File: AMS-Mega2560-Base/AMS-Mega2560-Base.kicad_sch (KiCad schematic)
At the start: 19 parts, among them J1 RTD1, J2 RTD2, J3 AdafruitUltimateGPS, J4 Sense, J5 Sense, P1 Power, P10 CONN_01X01, P11 CONN_01X01, P12 CONN_01X01, P13 CONN_01X01, P2 Analog, P3 Analog, P4 Digital, P5 PWM, P6 PWM, P7 Communication, P8 CONN_01X01, P9 CONN_01X01

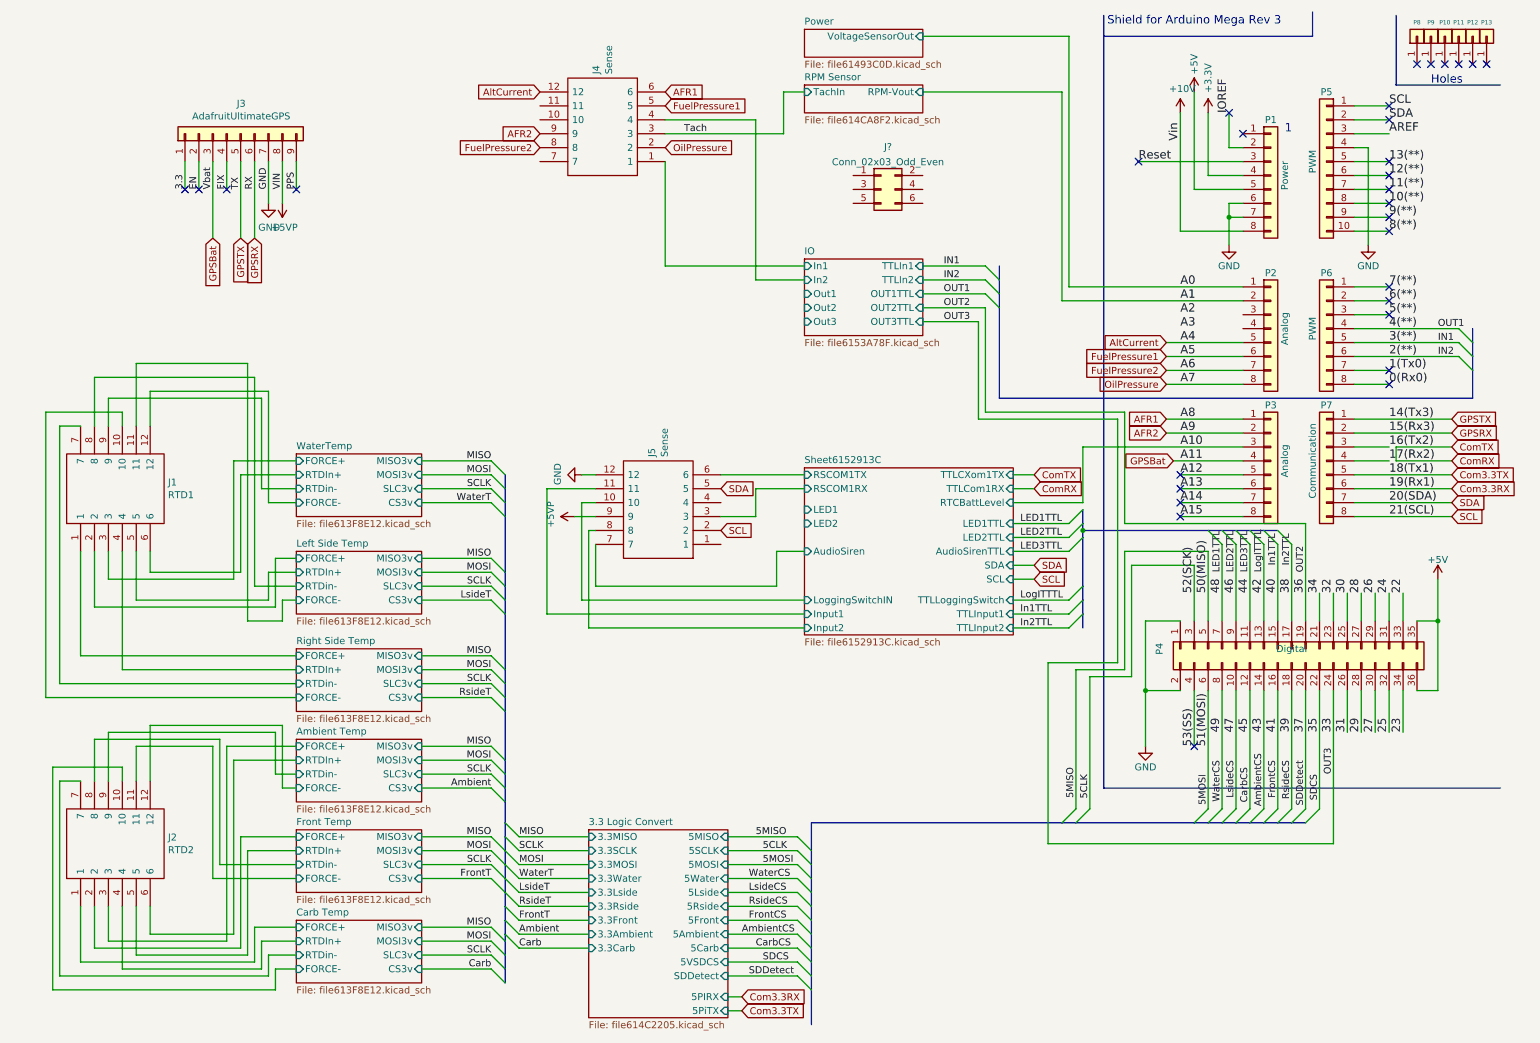
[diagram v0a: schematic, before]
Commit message: BaseBoard fixes and updates. doing schematic work.
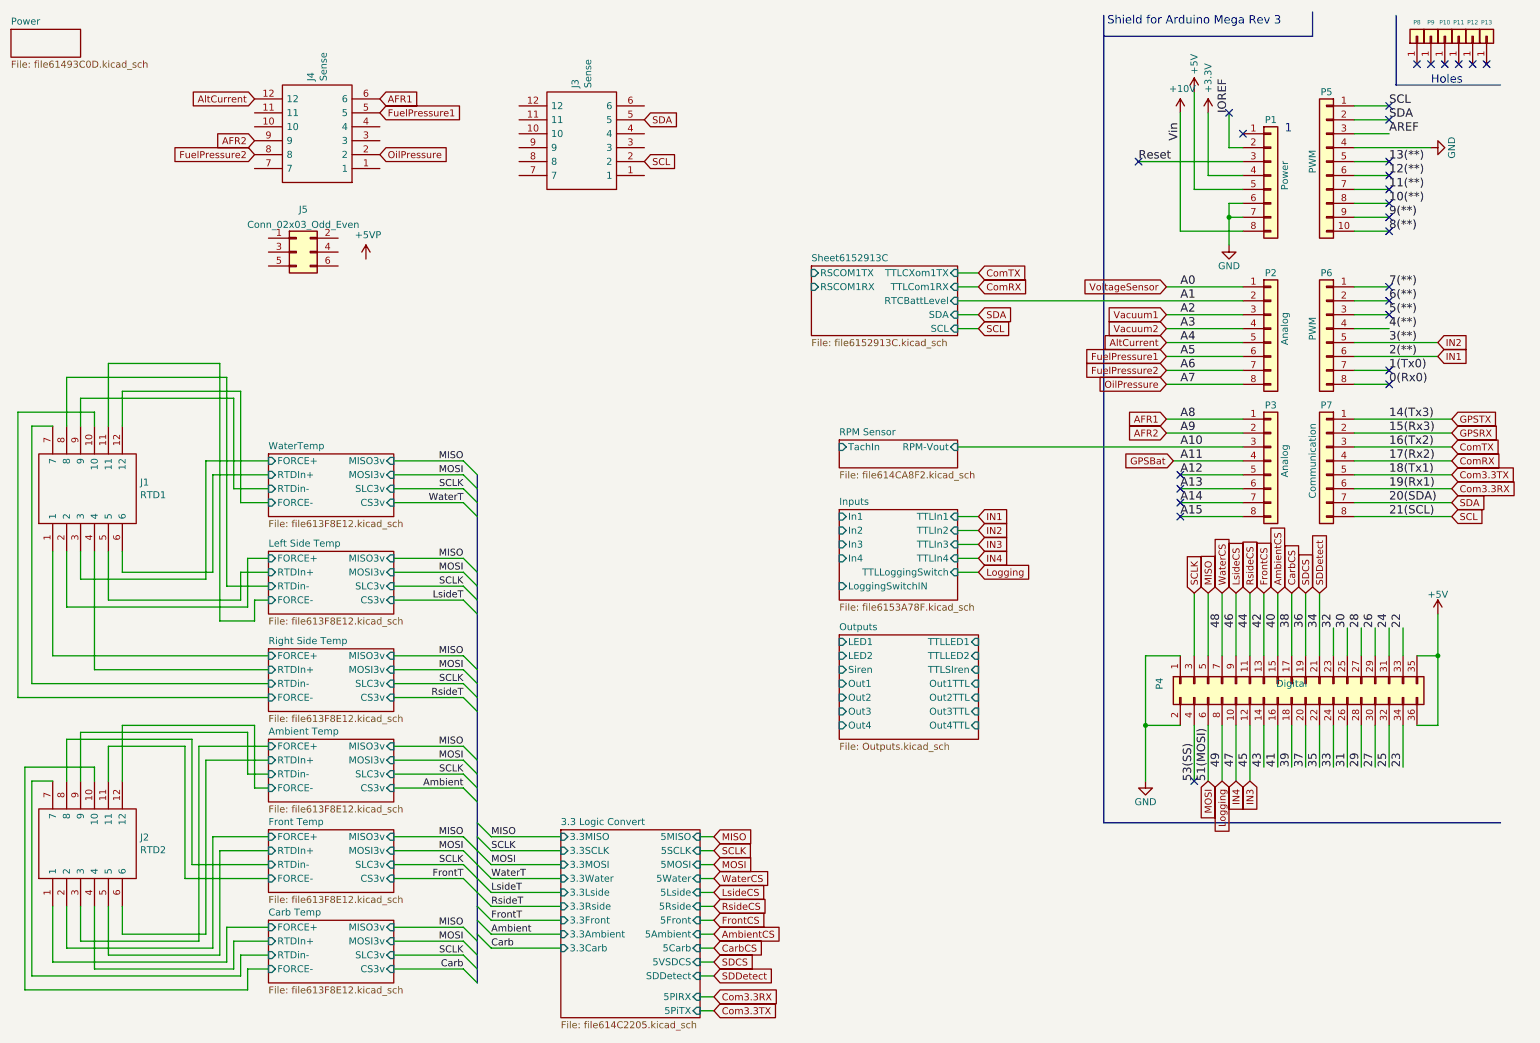
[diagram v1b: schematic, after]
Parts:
- removed J3: AdafruitUltimateGPS, Connector_PinSocket_2.54mm:PinSocket_1x09_P2.54mm_Vertical, symbol Connector_Generic:Conn_01x09
- gave numbers to parts that had none: 1
- renumbered J5 to J3
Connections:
- net 17(Rx2) is gone; now on net ComRX: P7.4 (Pin_4)
- net 50(MISO) is gone; now on net MISO: P4.5 (Pin_5)
- net 51(MOSI) is gone; now on net MOSI: P4.6 (Pin_6)
- net 52(SCK) is gone; now on net SCLK: P4.3 (Pin_3)
- net +5VP: no longer J3.9
- net GND: no longer J3.12
- net Inputs/In1: no longer J4.1
- net Inputs/In2: no longer J4.4
- net Sheet6152913C/RSCOM1RX: no longer J3.3
- net Sheet6152913C/RSCOM1TX: no longer J3.6
- net Vacuum1: now reaches P2.3 (Pin_3)
- net Vacuum2: now reaches P2.4 (Pin_4)
- net 16(Tx2) renamed ComTX
- net 2(**) renamed IN1
- net 3(**) renamed IN2
- net 34 renamed SDDetect
- net 36 renamed SDCS
- net 38 renamed CarbCS
- net 40 renamed AmbientCS
- net 42 renamed FrontCS
- net 44 renamed RsideCS
- net 45 renamed IN3
- net 46 renamed LsideCS
- net 47 renamed IN4
- net 48 renamed WaterCS
- net 49 renamed Logging
- net A0 renamed VoltageSensor
- net Sheet6152913C/AudioSiren: no longer names the net of J3.7
- net Sheet6152913C/Input1: no longer names the net of J3.11
- net Sheet6152913C/Input2: no longer names the net of J3.8
- net Sheet6152913C/LoggingSwitchIN: no longer names the net of J3.10
- net Tach: no longer names the net of J4.3
- no-connect marks 31 -> 27
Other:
- sheet IO renamed Inputs
- added sheet Outputs (Outputs.kicad_sch)
- sheet Inputs ports: added In3, In4, LoggingSwitchIN, TTLIn3, TTLIn4, TTLLoggingSwitch; removed OUT1TTL, OUT2TTL, OUT3TTL, Out1, Out2, Out3
- sheet Power ports: added none; removed VoltageSensorOut
- sheet Sheet6152913C ports: added none; removed AudioSiren, AudioSirenTTL, Input1, Input2, LED1, LED1TTL, LED2, LED2TTL, LoggingSwitchIN, TTLInput1, TTLInput2, TTLLoggingSwitch
- moved on the sheet: J1, J2, J3, J4, J5, P4
